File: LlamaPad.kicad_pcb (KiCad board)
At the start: 2 copper layers, 84.2 x 136.7 mm, 55 parts, among them J1 Conn_01x04_Pin, SW1 SW_Push, SW10 SW_Push, SW11 SW_Push, SW12 SW_Push, SW13 SW_Push, SW14 SW_Push, SW15 SW_Push, SW16 SW_Push, SW2 SW_Push, SW3 SW_Push, SW4 SW_Push, SW5 SW_Push, SW6 SW_Push, SW7 SW_Push, SW8 SW_Push, SW9 SW_Push

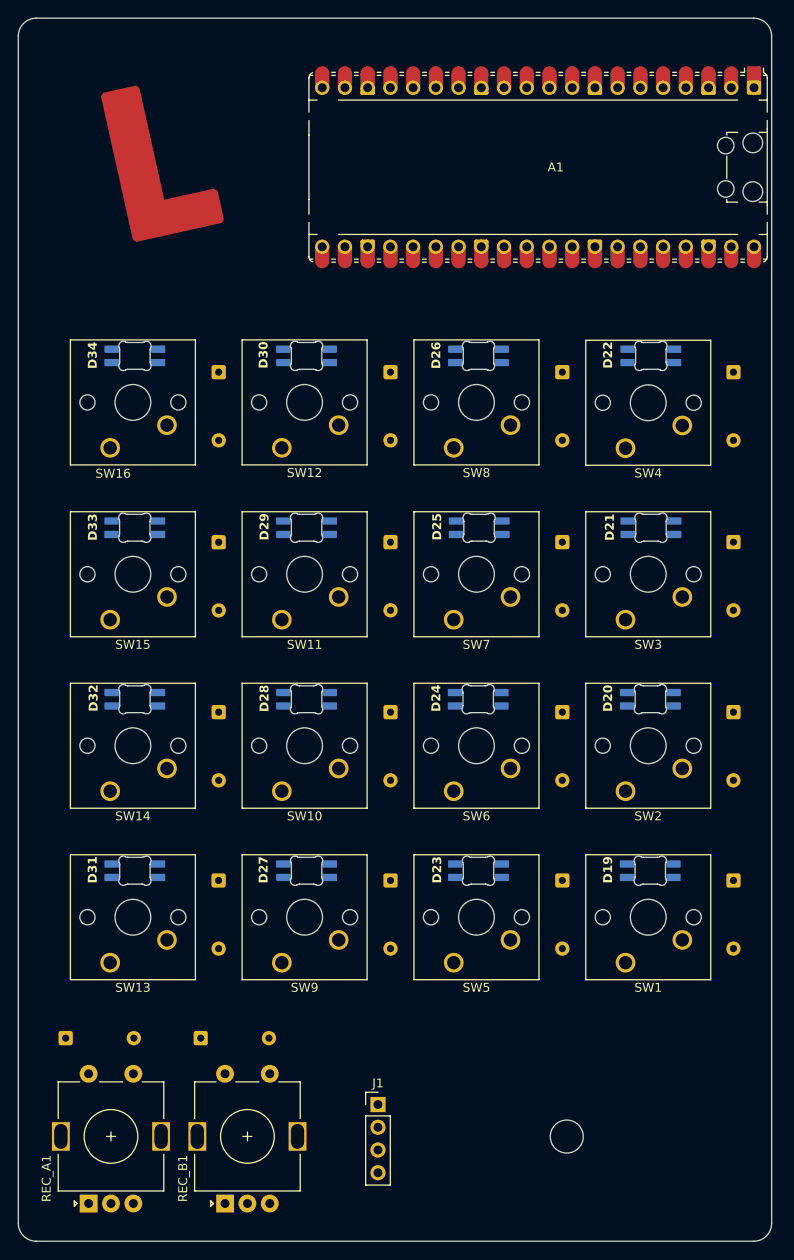
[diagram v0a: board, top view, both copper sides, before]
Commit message: feat: route the pcb and change schematic to be easier
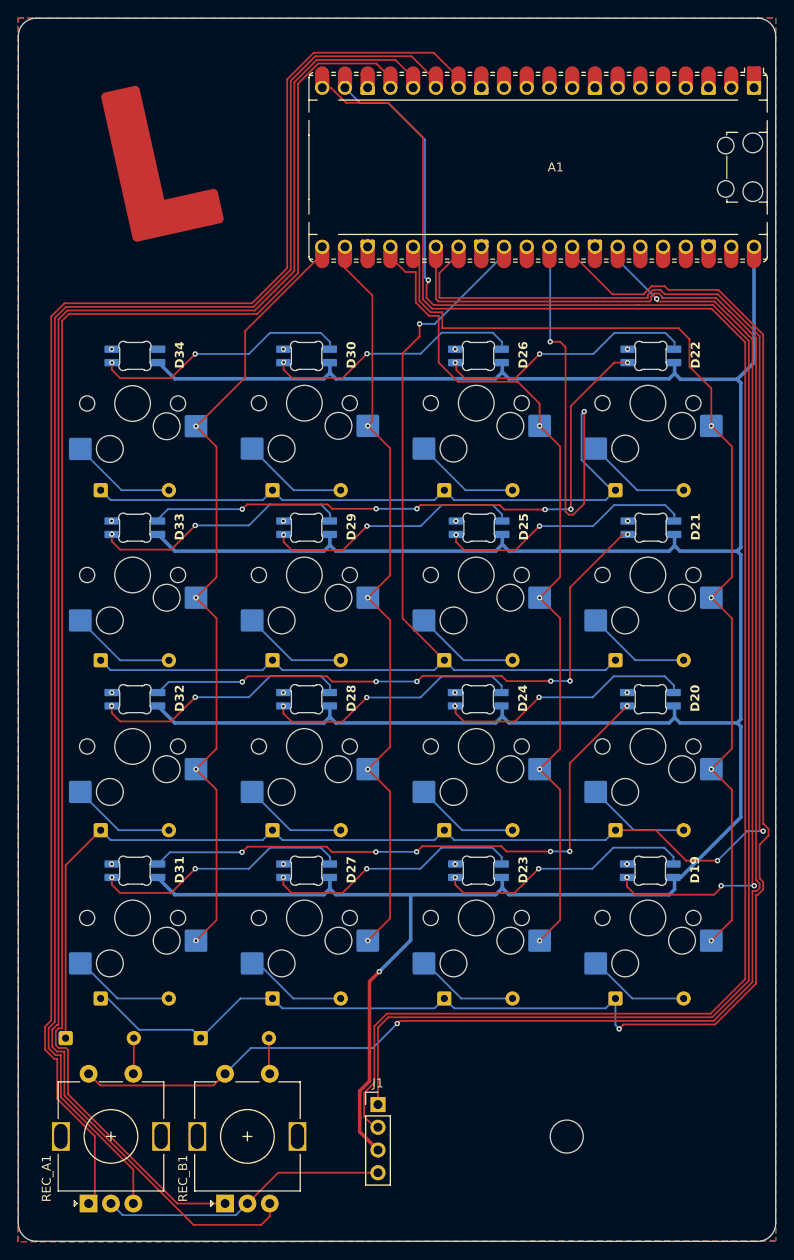
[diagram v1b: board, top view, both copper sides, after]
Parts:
- D19, D20, D21, D22, D23, D24, D25, D26, D27, D28, D29, D30, D31, D32, D33, D34: footprint HackPad:SK6812MINI-E_fixed -> Llama_Other:SK6812MINI-E_fixed
- REC_A1, REC_B1: footprint HackPad:RotaryEncoder_Alps_EC11E-Switch_Vertical_H20mm -> RotaryEncoder:RotaryEncoder_Alps_EC11E-Switch_Vertical_H20mm
- SW1, SW10, SW11, SW12, SW13, SW14, SW15, SW16, SW2, SW3, SW4, SW5, SW6, SW7, SW8, SW9: footprint Button_Switch_Keyboard:SW_Cherry_MX_1.00u_PCB -> Switch_MX_Hotswap:MX-Hotswap-1U; moved to B.Cu
- moved SW13 60.3 mm to (149.8, 133.0), turned to 0 degrees
- moved SW14 60.3 mm to (149.8, 113.8), turned to 0 degrees
- moved SW15 60.3 mm to (149.8, 94.7), turned to 0 degrees
- moved SW16 60.3 mm to (149.8, 75.5), turned to 0 degrees
- moved SW1 55.3 mm to (92.2, 133.0), turned to 0 degrees
- moved SW2 55.3 mm to (92.2, 113.8), turned to 0 degrees
- moved SW3 55.3 mm to (92.2, 94.7), turned to 0 degrees
- moved SW4 55.3 mm to (92.2, 75.5), turned to 0 degrees
- moved SW10 22.3 mm to (130.6, 113.8), turned to 0 degrees
- moved SW12 22.3 mm to (130.6, 75.5), turned to 0 degrees
- moved SW9 22.3 mm to (130.6, 133.0), turned to 0 degrees
- moved SW11 22.3 mm to (130.6, 94.7), turned to 0 degrees
- moved D13 18.7 mm to (146.2, 85.2), turned to 0 degrees
- moved D14 18.7 mm to (146.2, 104.2), turned to 0 degrees
- moved D15 18.7 mm to (146.2, 123.2), turned to 0 degrees
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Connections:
- A1 pad 1: ROW0 -> unconnected-(A1-GPIO0-Pad1)
- A1 pad 10: COL3 -> unconnected-(A1-GPIO7-Pad10)
- A1 pad 11: COL4 -> unconnected-(A1-GPIO8-Pad11)
- A1 pad 12: REC_A1 -> unconnected-(A1-GPIO9-Pad12)
- A1 pad 15: REC_B1 -> REC_A1
- A1 pad 16: REC_B2 -> REC_B1
- A1 pad 17: ARGB_DATA -> REC_B2
- A1 pad 2: ROW1 -> unconnected-(A1-GPIO1-Pad2)
- A1 pad 21: unconnected-(A1-GPIO16-Pad21) -> COL0
- A1 pad 22: unconnected-(A1-GPIO17-Pad22)_1 -> COL1
- A1 pad 24: unconnected-(A1-GPIO18-Pad24)_1 -> COL2
- A1 pad 25: unconnected-(A1-GPIO19-Pad25) -> COL3
- A1 pad 26: unconnected-(A1-GPIO20-Pad26) -> COL4
- A1 pad 27: unconnected-(A1-GPIO21-Pad27) -> ROW1
- A1 pad 29: unconnected-(A1-GPIO22-Pad29)_1 -> ROW2
- A1 pad 31: unconnected-(A1-GPIO26_ADC0-Pad31) -> ROW3
- A1 pad 32: unconnected-(A1-GPIO27_ADC1-Pad32)_1 -> ROW0
- A1 pad 34: unconnected-(A1-GPIO28_ADC2-Pad34)_1 -> ARGB_DATA
- A1 pad 4: ROW2 -> unconnected-(A1-GPIO2-Pad4)
- A1 pad 5: ROW3 -> unconnected-(A1-GPIO3-Pad5)
- A1 pad 6: COL0 -> unconnected-(A1-GPIO4-Pad6)
- A1 pad 7: COL1 -> unconnected-(A1-GPIO5-Pad7)
- A1 pad 9: COL2 -> unconnected-(A1-GPIO6-Pad9)
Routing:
- net VCC: track 0.00 -> 383.1 mm, vias 0 -> 1
- net ROW1: track 0.00 -> 204.3 mm, vias 0 -> 2
- net OLED_SCL: track 0.00 -> 197.1 mm
- net COL4: track 0.00 -> 196.0 mm, vias 0 -> 1
- net OLED_SDA: track 0.00 -> 192.9 mm, vias 0 -> 1
- net REC_B1: track 0.00 -> 184.9 mm
- net ROW0: track 0.00 -> 183.7 mm, vias 0 -> 1
- net REC_A2: track 0.00 -> 174.6 mm
- net REC_B2: track 0.00 -> 173.4 mm
- net REC_A1: track 0.00 -> 171.7 mm
- net ROW3: track 0.00 -> 115.0 mm, vias 0 -> 2
- net ROW2: track 0.00 -> 114.1 mm, vias 0 -> 1
- net COL3: track 0.00 -> 113.0 mm, vias 0 -> 4
- net ARGB_DATA: track 0.00 -> 97.6 mm, vias 0 -> 4
- net COL2: track 0.00 -> 95.4 mm, vias 0 -> 4
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- added copper zone on B.Cu, net GND
- added copper zone on F.Cu, net GND
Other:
- board size 84.2 x 136.7 mm -> 84.7 x 136.7 mm
